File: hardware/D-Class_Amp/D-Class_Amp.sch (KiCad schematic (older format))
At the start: 25 parts, among them J101 Barrel_Jack_MountingPin, J102 AudioJack2, U101 NCP1117-12_TO252, U102 MCP1799T-5002H_TT

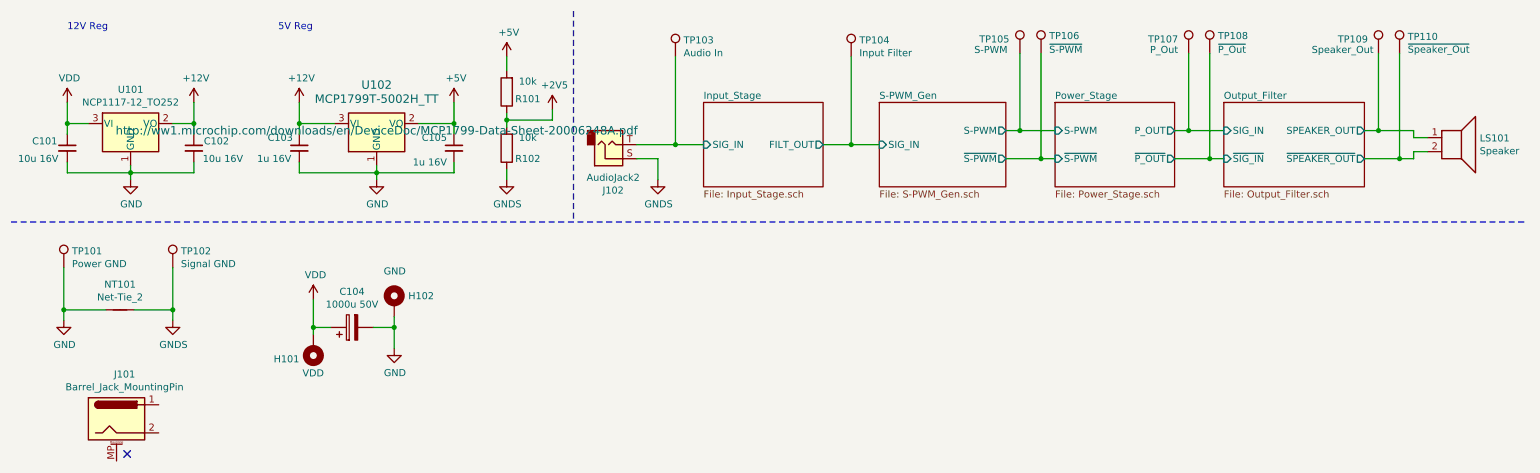
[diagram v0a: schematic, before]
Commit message: updated the BOM
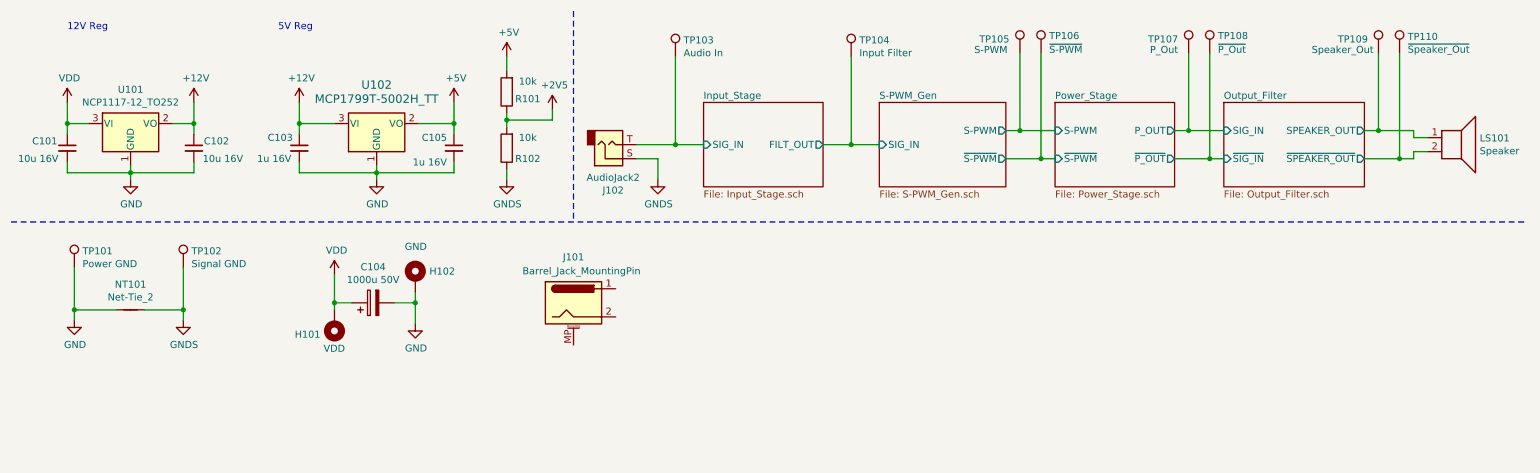
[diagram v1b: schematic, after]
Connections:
- no-connect marks 1 -> 0
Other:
- moved on the sheet: C104, H101, H102, J101, NT101, TP101, TP102
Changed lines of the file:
@@
 L power:GNDS #PWR0104
 U 1 1 612A4FBB
-P 1600 2675
-F 0 "#PWR0104" H 1600 2425 50  0001 C CNN
-F 1 "GNDS" H 1605 2502 50  0000 C CNN
-F 2 "" H 1600 2675 50  0001 C CNN
-F 3 "" H 1600 2675 50  0001 C CNN
-	1    1600 2675
+P 1675 2675
+F 0 "#PWR0104" H 1675 2425 50  0001 C CNN
+F 1 "GNDS" H 1680 2502 50  0000 C CNN
+F 2 "" H 1675 2675 50  0001 C CNN
+F 3 "" H 1675 2675 50  0001 C CNN
+	1    1675 2675
 	1    0    0    -1
 $EndComp
@@
 L power:GND #PWR0101
 U 1 1 612A56C1
-P 825 2675
-F 0 "#PWR0101" H 825 2425 50  0001 C CNN
-F 1 "GND" H 830 2502 50  0000 C CNN
-F 2 "" H 825 2675 50  0001 C CNN
-F 3 "" H 825 2675 50  0001 C CNN
-	1    825  2675
+P 900 2675
+F 0 "#PWR0101" H 900 2425 50  0001 C CNN
+F 1 "GND" H 905 2502 50  0000 C CNN
+F 2 "" H 900 2675 50  0001 C CNN
+F 3 "" H 900 2675 50  0001 C CNN
+	1    900  2675
 	1    0    0    -1
 $EndComp
@@
 L Device:Net-Tie_2 NT101
 U 1 1 612A676E
-P 1225 2600
-F 0 "NT101" H 1225 2781 50  0000 C CNN
-F 1 "Net-Tie_2" H 1225 2690 50  0000 C CNN
-F 2 "" H 1225 2600 50  0001 C CNN
-F 3 "~" H 1225 2600 50  0001 C CNN
-	1    1225 2600
-	1    0    0    -1
-$EndComp
-Wire Wire Line
-	825  2675 825  2600
-Wire Wire Line
-	825  2600 1125 2600
-Wire Wire Line
-	1325 2600 1600 2600
-Wire Wire Line
-	1600 2600 1600 2675
+P 1300 2600
+F 0 "NT101" H 1300 2781 50  0000 C CNN
+F 1 "Net-Tie_2" H 1300 2690 50  0000 C CNN
+F 2 "" H 1300 2600 50  0001 C CNN
+F 3 "~" H 1300 2600 50  0001 C CNN
+	1    1300 2600
+	1    0    0    -1
+$EndComp
+Wire Wire Line
+	900  2675 900  2600
+Wire Wire Line
+	900  2600 1200 2600
+Wire Wire Line
+	1400 2600 1675 2600
+Wire Wire Line
+	1675 2600 1675 2675
 $Comp
 L Connector:TestPoint TP103
@@
 F 1 "MCP1799T-5002H_TT" H 3050 1550 60  0000 C CNN
 F 2 "Package_TO_SOT_SMD:SOT-23_Handsoldering" H 3850 1565 60  0001 C CNN
-F 3 "http://ww1.microchip.com/downloads/en/DeviceDoc/MCP1799-Data-Sheet-20006248A.pdf" H 3050 1325 60  0000 C CNN
+F 3 "http://ww1.microchip.com/downloads/en/DeviceDoc/MCP1799-Data-Sheet-20006248A.pdf" H 3050 1325 60  0001 C CNN
 F 4 "0.62" H 3050 1325 50  0001 C CNN "DigiKey Price"
 F 5 "MCP1799T-5002H/TT" H 3050 1325 50  0001 C CNN "Part Number"
@@
 L Connector:TestPoint TP101
 U 1 1 6113B2E7
-P 825 2300
-F 0 "TP101" H 883 2418 50  0000 L CNN
-F 1 "Power GND" H 883 2327 50  0000 L CNN
-F 2 "TestPoint:TestPoint_THTPad_D2.0mm_Drill1.0mm" H 1025 2300 50  0001 C CNN
-F 3 "~" H 1025 2300 50  0001 C CNN
-	1    825  2300
+P 900 2300
+F 0 "TP101" H 958 2418 50  0000 L CNN
+F 1 "Power GND" H 958 2327 50  0000 L CNN
+F 2 "TestPoint:TestPoint_THTPad_D2.0mm_Drill1.0mm" H 1100 2300 50  0001 C CNN
+F 3 "~" H 1100 2300 50  0001 C CNN
+	1    900  2300
 	1    0    0    -1
 $EndComp
@@
 L Connector:TestPoint TP102
 U 1 1 6113B863
-P 1600 2300
-F 0 "TP102" H 1658 2418 50  0000 L CNN
-F 1 "Signal GND" H 1658 2327 50  0000 L CNN
-F 2 "TestPoint:TestPoint_THTPad_D2.0mm_Drill1.0mm" H 1800 2300 50  0001 C CNN
-F 3 "~" H 1800 2300 50  0001 C CNN
-	1    1600 2300
-	1    0    0    -1
-$EndComp
-Wire Wire Line
-	825  2300 825  2600
-Connection ~ 825  2600
-Wire Wire Line
-	1600 2300 1600 2600
-Connection ~ 1600 2600
+P 1675 2300
+F 0 "TP102" H 1733 2418 50  0000 L CNN
+F 1 "Signal GND" H 1733 2327 50  0000 L CNN
+F 2 "TestPoint:TestPoint_THTPad_D2.0mm_Drill1.0mm" H 1875 2300 50  0001 C CNN
+F 3 "~" H 1875 2300 50  0001 C CNN
+	1    1675 2300
+	1    0    0    -1
+$EndComp
+Wire Wire Line
+	900  2300 900  2600
+Connection ~ 900  2600
+Wire Wire Line
+	1675 2300 1675 2600
+Connection ~ 1675 2600
 Wire Wire Line
 	3975 1600 3975 1675
@@
 	3975 1250 4300 1250
 $Comp
+L Mechanical:MountingHole_Pad H102
+U 1 1 6126D650
+P 3325 2375
+F 0 "H102" H 3425 2424 50  0000 L CNN
+F 1 "GND" H 3250 2600 50  0000 L CNN
+F 2 "" H 3325 2375 50  0001 C CNN
+F 3 "~" H 3325 2375 50  0001 C CNN
+	1    3325 2375
+	1    0    0    -1
+$EndComp
+$Comp
+L power:GND #PWR0109
+U 1 1 6127C8B5
+P 3325 2700
+F 0 "#PWR0109" H 3325 2450 50  0001 C CNN
+F 1 "GND" H 3330 2527 50  0000 C CNN
+F 2 "" H 3325 2700 50  0001 C CNN
+F 3 "" H 3325 2700 50  0001 C CNN
+	1    3325 2700
+	1    0    0    -1
+$EndComp
+Wire Wire Line
+	3325 2700 3325 2550
+$Comp
+L Device:CP C104
+U 1 1 6127F37C
+P 3025 2550
+F 0 "C104" V 3280 2550 50  0000 C CNN
+F 1 "1000u 50V" V 3189 2550 50  0000 C CNN
+F 2 "Capacitor_THT:CP_Radial_D10.0mm_P5.00mm" H 3063 2400 50  0001 C CNN
+F 3 "~" H 3025 2550 50  0001 C CNN
+F 4 "1" H 3025 2550 50  0001 C CNN "DigiKey Price"
+	1    3025 2550
+	0    -1   -1   0
+$EndComp
+Wire Wire Line
+	3175 2550 3325 2550
+Connection ~ 3325 2550
+Wire Wire Line
+	3325 2550 3325 2475
+$Comp
+L power:VDD #PWR?
+U 1 1 612997D9
+P 2750 2350
+AR Path="/610497A4/612997D9" Ref="#PWR?"  Part="1"
+AR Path="/612997D9" Ref="#PWR0107"  Part="1"
+F 0 "#PWR0107" H 2750 2200 50  0001 C CNN
+F 1 "VDD" H 2765 2523 50  0000 C CNN
+F 2 "" H 2750 2350 50  0001 C CNN
+F 3 "" H 2750 2350 50  0001 C CNN
+	1    2750 2350
+	1    0    0    -1
+$EndComp
+$Comp
+L Mechanical:MountingHole_Pad H101
+U 1 1 6126CC33
+P 2750 2700
+F 0 "H101" H 2850 2775 50  0000 L CNN
+F 1 "VDD" H 2675 2875 50  0000 L CNN
+F 2 "" H 2750 2700 50  0001 C CNN
+F 3 "~" H 2750 2700 50  0001 C CNN
+	1    2750 2700
+	-1   0    0    1
+$EndComp
+Wire Wire Line
+	2750 2350 2750 2550
+Connection ~ 2750 2550
+Wire Wire Line
+	2750 2600 2750 2550
+Wire Wire Line
+	2750 2550 2875 2550
+$Comp
 L Connector:Barrel_Jack_MountingPin J101
 U 1 1 612622C7
-P 1200 3375
-F 0 "J101" H 1257 3692 50  0000 C CNN
-F 1 "Barrel_Jack_MountingPin" H 1257 3601 50  0000 C CNN
-F 2 "" H 1250 3335 50  0001 C CNN
-F 3 "~" H 1250 3335 50  0001 C CNN
-	1    1200 3375
-	1    0    0    -1
-$EndComp
-NoConn ~ 1275 3625
-$Comp
-L Mechanical:MountingHole_Pad H102
-U 1 1 6126D650
-P 3175 2550
-F 0 "H102" H 3275 2599 50  0000 L CNN
-F 1 "GND" H 3100 2775 50  0000 L CNN
-F 2 "" H 3175 2550 50  0001 C CNN
-F 3 "~" H 3175 2550 50  0001 C CNN
-	1    3175 2550
-	1    0    0    -1
-$EndComp
-$Comp
-L power:GND #PWR0109
-U 1 1 6127C8B5
-P 3175 2875
-F 0 "#PWR0109" H 3175 2625 50  0001 C CNN
-F 1 "GND" H 3180 2702 50  0000 C CNN
-F 2 "" H 3175 2875 50  0001 C CNN
-F 3 "" H 3175 2875 50  0001 C CNN
-	1    3175 2875
-	1    0    0    -1
-$EndComp
-Wire Wire Line
-	3175 2875 3175 2725
-$Comp
-L Device:CP C104
-U 1 1 6127F37C
-P 2875 2725
-F 0 "C104" V 3130 2725 50  0000 C CNN
-F 1 "1000u 50V" V 3039 2725 50  0000 C CNN
-F 2 "Capacitor_THT:CP_Radial_D10.0mm_P5.00mm" H 2913 2575 50  0001 C CNN
-F 3 "~" H 2875 2725 50  0001 C CNN
-F 4 "1" H 2875 2725 50  0001 C CNN "DigiKey Price"
-	1    2875 2725
-	0    -1   -1   0
-$EndComp
-Wire Wire Line
-	3025 2725 3175 2725
-Connection ~ 3175 2725
-Wire Wire Line
-	3175 2725 3175 2650
-$Comp
-L power:VDD #PWR?
-U 1 1 612997D9
-P 2600 2525
-AR Path="/610497A4/612997D9" Ref="#PWR?"  Part="1"
-AR Path="/612997D9" Ref="#PWR0107"  Part="1"
-F 0 "#PWR0107" H 2600 2375 50  0001 C CNN
-F 1 "VDD" H 2615 2698 50  0000 C CNN
-F 2 "" H 2600 2525 50  0001 C CNN
-F 3 "" H 2600 2525 50  0001 C CNN
-	1    2600 2525
-	1    0    0    -1
-$EndComp
-$Comp
-L Mechanical:MountingHole_Pad H101
-U 1 1 6126CC33
-P 2600 2875
-F 0 "H101" H 2700 2950 50  0000 L CNN
-F 1 "VDD" H 2525 3050 50  0000 L CNN
-F 2 "" H 2600 2875 50  0001 C CNN
-F 3 "~" H 2600 2875 50  0001 C CNN
-	1    2600 2875
-	-1   0    0    1
-$EndComp
-Wire Wire Line
-	2600 2525 2600 2725
-Connection ~ 2600 2725
-Wire Wire Line
-	2600 2775 2600 2725
-Wire Wire Line
-	2600 2725 2725 2725
+P 4450 2550
+F 0 "J101" H 4450 2875 50  0000 C CNN
+F 1 "Barrel_Jack_MountingPin" H 4507 2776 50  0000 C CNN
+F 2 "" H 4500 2510 50  0001 C CNN
+F 3 "~" H 4500 2510 50  0001 C CNN
+	1    4450 2550
+	1    0    0    -1
+$EndComp
 $EndSCHEMATC
